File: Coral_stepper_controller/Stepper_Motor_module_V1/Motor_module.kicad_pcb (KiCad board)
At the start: 2 copper layers, 28.5 x 40 mm, 34 parts, among them J1 Limit Switch, J2 Limit Switch, J3 Limit Switch, J4 Limit Switch, J5 Conn_01x08_Male, J6 Conn_01x04_Male, J7 Conn_01x08_Female, J8 Conn_01x08_Female, SW1 SW_Push, U1 STM32F031F6Px, U3 THVD1439DR, Y1 8MHz

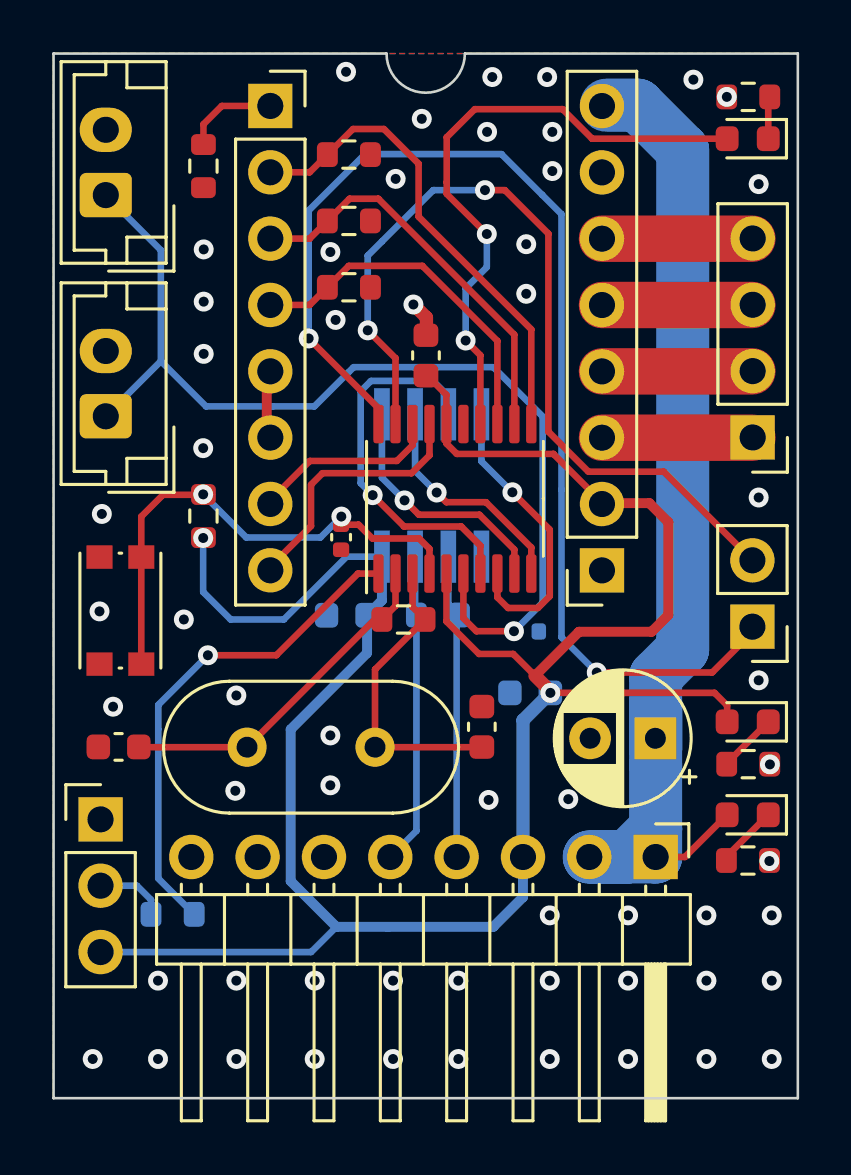
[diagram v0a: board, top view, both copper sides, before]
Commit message: udated by FZ
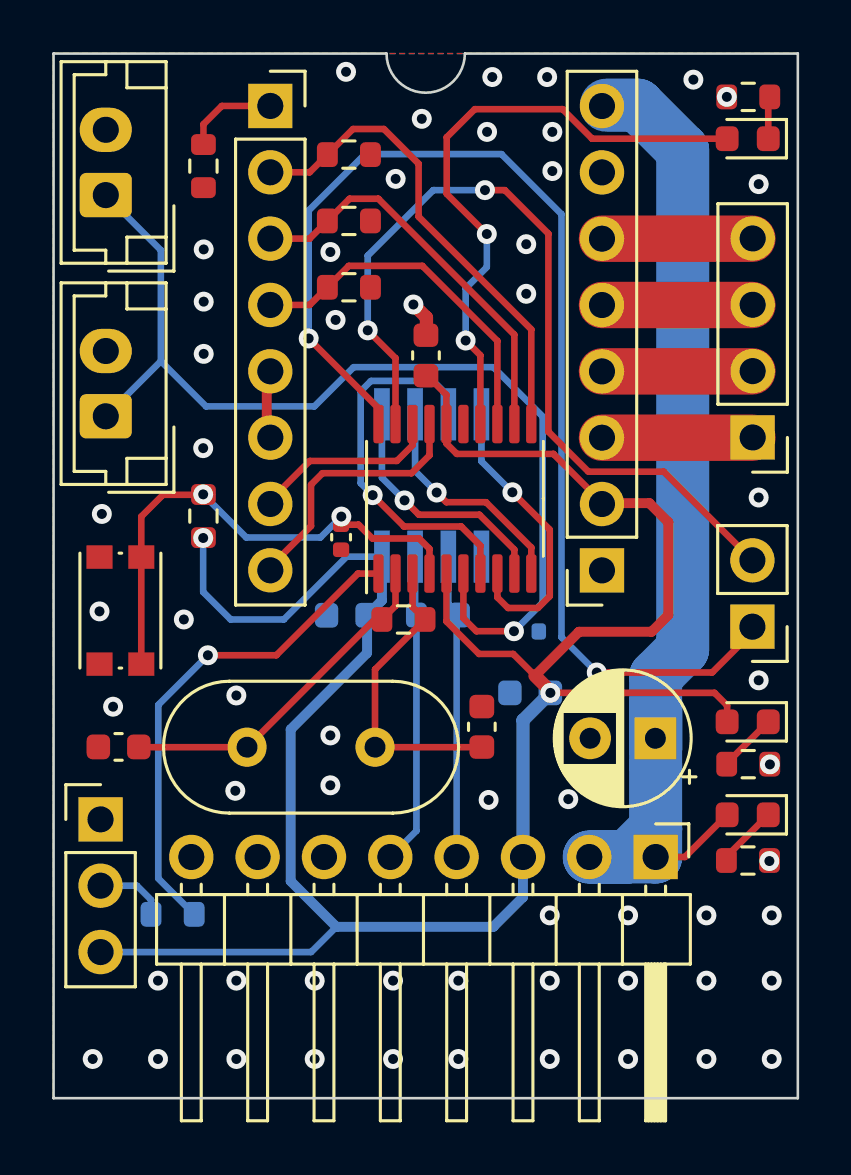
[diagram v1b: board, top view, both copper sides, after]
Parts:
- U1: value STM32F031F6Px -> STM32F031F6P6
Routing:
- net /SWCLK: track 45.7 -> 44.9 mm
- net /RS485_DE: track 14.6 -> 13.9 mm
